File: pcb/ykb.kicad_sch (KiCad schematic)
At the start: 90 parts, among them J1 Conn_01x08_Socket, U1 Helios

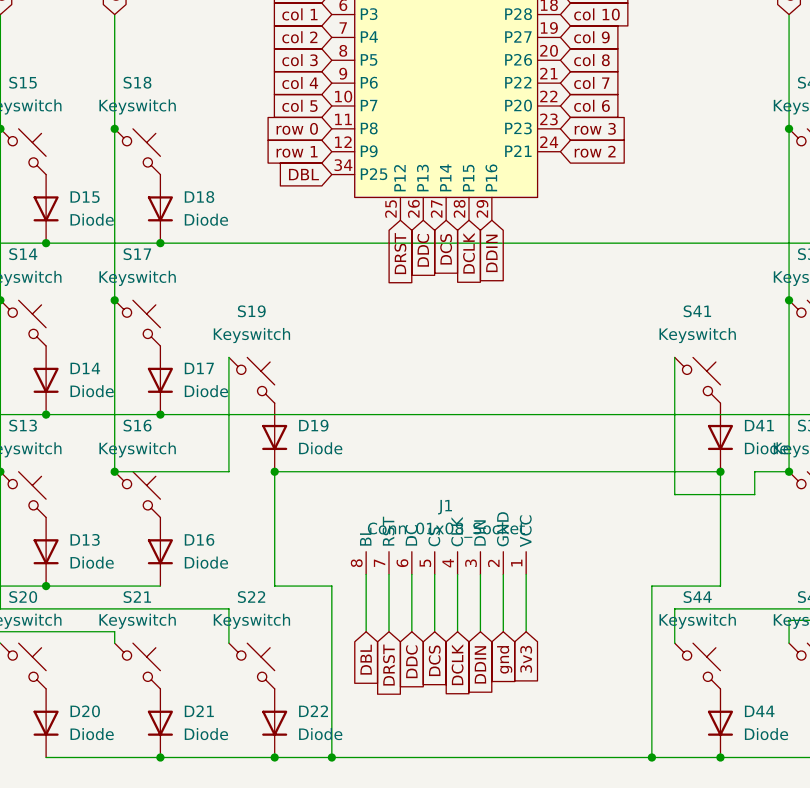
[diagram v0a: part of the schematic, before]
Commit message: all done other than mounting holes :3
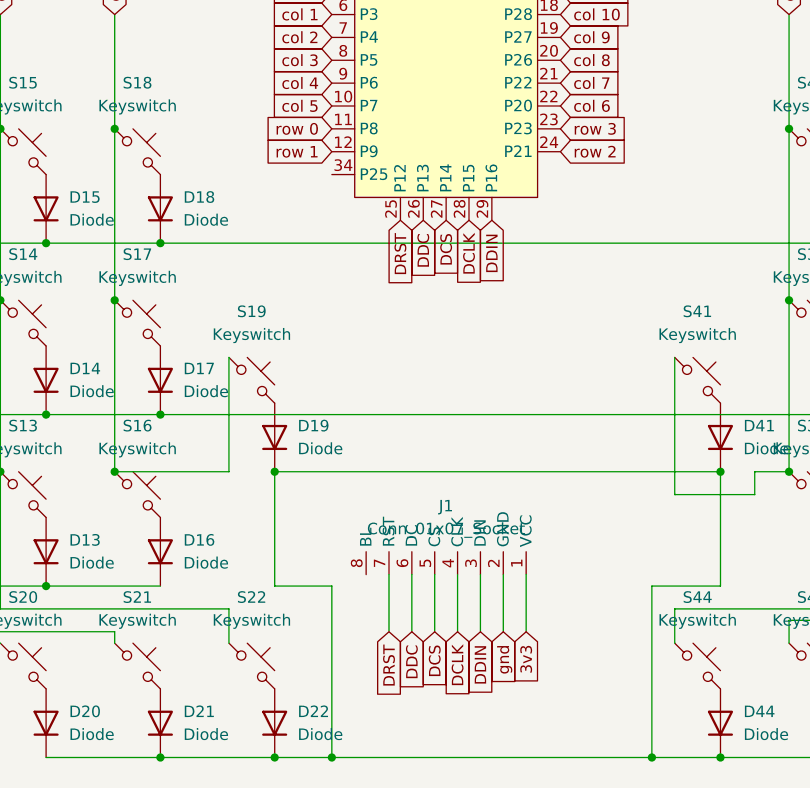
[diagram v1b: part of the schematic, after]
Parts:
- J1: value Conn_01x08_Socket -> Conn_01x07_Socket; footprint Connector_PinHeader_2.54mm:PinHeader_1x08_P2.54mm_Vertical -> Connector_PinHeader_2.54mm:PinHeader_1x07_P2.54mm_Vertical
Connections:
- net DBL: no longer names the net of U1.34 (P25)
- net DBL: no longer J1.8 (BL)
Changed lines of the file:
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@@
 	(wire
 		(pts
-			(xy 143.51 100.33) (xy 143.51 106.68)
-		)
-		(stroke
-			(width 0)
-			(type default)
-		)
-	)
-	(wire
-		(pts
 			(xy 102.87 69.85) (xy 102.87 88.9)
 		)
@@
 		)
 	)
-	(global_label "DBL"
-		(shape input)
-		(at 143.51 106.68 270)
-		(fields_autoplaced yes)
-		(effects
-			(font
-				(size 1.27 1.27)
-			)
-			(justify right)
-		)
-		(property "Intersheetrefs" "${INTERSHEET_REFS}"
-			(at 143.51 113.2333 90)
-			(effects
-				(font
-					(size 1.27 1.27)
-				)
-				(justify right)
-				(hide yes)
-			)
-		)
-	)
 	(global_label "col 2"
 		(shape input)
@@
 		)
 	)
-	(global_label "DBL"
-		(shape input)
-		(at 139.7 55.88 180)
-		(fields_autoplaced yes)
-		(effects
-			(font
-				(size 1.27 1.27)
-			)
-			(justify right)
-		)
-		(property "Intersheetrefs" "${INTERSHEET_REFS}"
-			(at 133.1467 55.88 0)
-			(effects
-				(font
-					(size 1.27 1.27)
-				)
-				(justify right)
-				(hide yes)
-			)
-		)
-	)
 	(global_label "col 10"
 		(shape input)
@@
 			)
 		)
-		(property "Value" "Conn_01x08_Socket"
+		(property "Value" "Conn_01x07_Socket"
 			(at 152.4 95.25 0)
 			(effects
@@
 			)
 		)
-		(property "Footprint" "Connector_PinHeader_2.54mm:PinHeader_1x08_P2.54mm_Vertical"
+		(property "Footprint" "Connector_PinHeader_2.54mm:PinHeader_1x07_P2.54mm_Vertical"
 			(at 147.32 100.33 0)
 			(effects
@@
 			)
 		)
-		(property "Description" "Generic connector, single row, 01x08, script generated"
+		(property "Description" "Generic connector, single row, 01x07, script generated"
 			(at 147.32 100.33 0)
 			(effects
